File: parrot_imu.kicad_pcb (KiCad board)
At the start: 2 copper layers, 50 x 100 mm, 29 parts, among them J1 Conn_01x02_Male, J2 SI-60062-F, J3 TB005-762-02BE, U1 TR05S3V3, U2 VR10S05, U3 Spark_fun_ICM-20948, U4 Teensy4.1, U5 TJA1441AT/0Z, U6 SOT_24-2BLY_STM

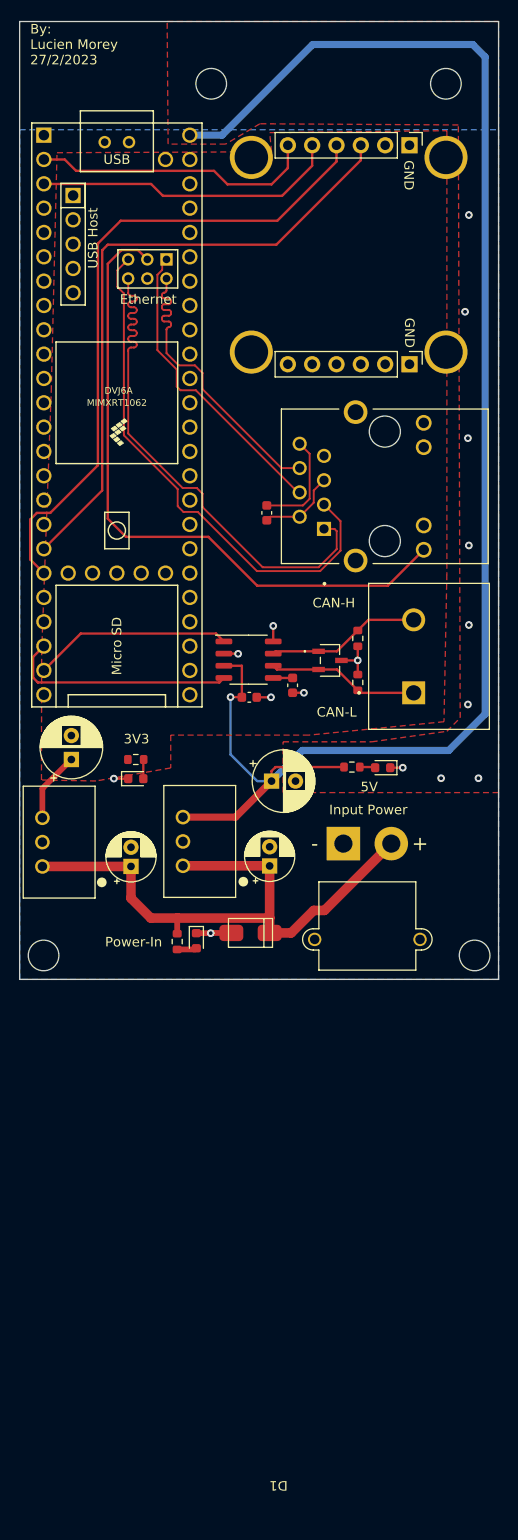
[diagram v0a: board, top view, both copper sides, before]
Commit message: update pcb
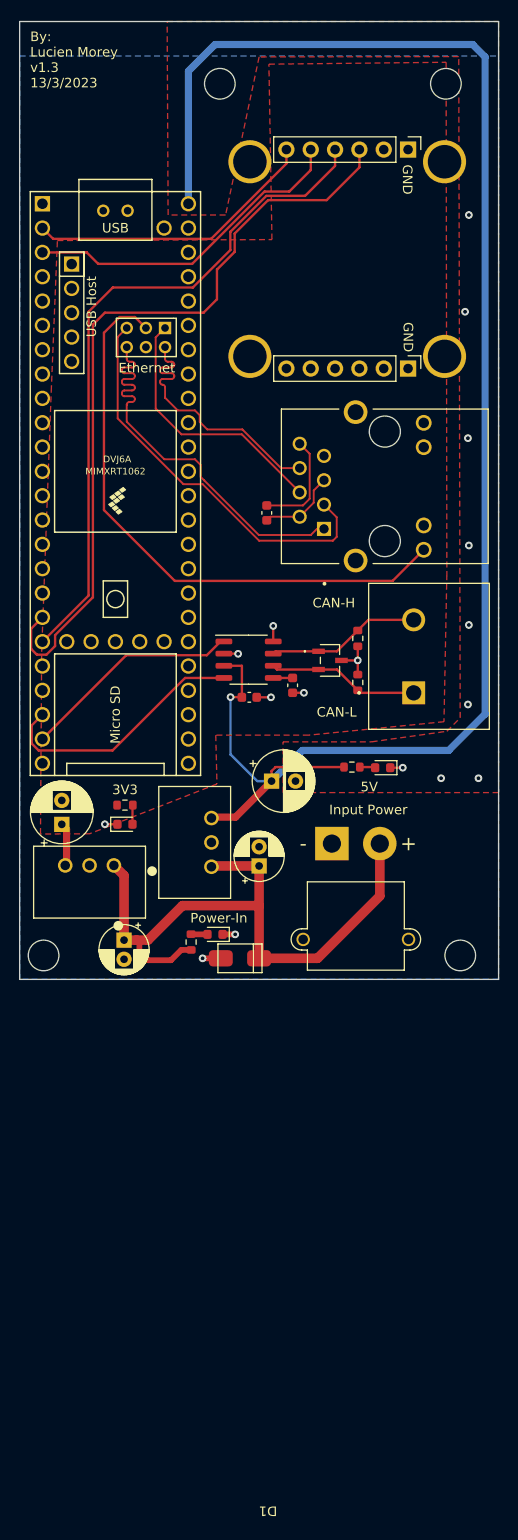
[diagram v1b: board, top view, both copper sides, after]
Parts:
- U6: value SOT_24-2BLY_STM -> ESDCAN24-2BLY
- moved H4 24.5 mm to (94.5, 55.5)
- moved H2 23.6 mm to (70.9, 55.5)
- moved C1 7.73 mm to (60.9, 144.9), turned to -90 degrees
- moved U4 7.16 mm to (60.0, 97.2)
- moved C4 6.84 mm to (54.4, 132.8)
- moved U1 5.49 mm to (57.3, 137.1), turned to 0 degrees
- moved D3 4.89 mm to (61.0, 132.8)
- moved R2 4.89 mm to (61.0, 130.8)
- moved U2 2.97 mm to (70.0, 134.7), turned to -90 degrees
- moved D1 2.87 mm to (73.0, 146.8)
- moved D2 2.06 mm to (70.4, 144.3), turned to 180 degrees
- moved H1 1.50 mm to (96.0, 146.5)
- moved R1 1.45 mm to (67.9, 145.1), turned to 90 degrees
- moved J1 1.20 mm to (82.6, 134.8)
- moved C2 1.10 mm to (75.0, 137.2)
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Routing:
- net /MOSI: track 66.1 -> 81.5 mm
- net /Eth_tx-: track 55.1 -> 42.1 mm
- net /Eth_tx+: track 54.8 -> 42.0 mm
- net +5V: track 166.5 -> 174.7 mm
- net /Eth_led: track 69.2 -> 61.8 mm
- net Net-(C1-Pad1): track 62.2 -> 66.7 mm
- net /Eth_rx+: track 31.9 -> 27.5 mm
- net /Eth_rx-: track 31.8 -> 27.4 mm
- net /Can_rx: track 24.1 -> 27.0 mm
- net +3.3V: track 9.36 -> 6.58 mm
- net /MISO: track 32.0 -> 34.7 mm
- net /Can_tx: track 20.7 -> 23.2 mm
- net /SCK: track 68.9 -> 71.3 mm
- net /CS: track 29.6 -> 30.7 mm
- net GND: track 27.8 -> 27.2 mm, vias 16 -> 17
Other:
- board text added: "By: Lucien Morey v1.3 13/3/2023"
- board text removed: "By: Lucien Morey 27/2/2023"
